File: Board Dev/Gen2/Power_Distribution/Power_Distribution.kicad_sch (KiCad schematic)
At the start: 27 parts, among them IC1 ACS713ELCTR-30A-T, IC2 ACS713ELCTR-30A-T, IC3 ACS713ELCTR-30A-T, IC4 ACS713ELCTR-30A-T, IC5 ACS713ELCTR-30A-T, IC6 ACS713ELCTR-30A-T, IC7 ACS713ELCTR-30A-T, IC8 ACS713ELCTR-30A-T, J1 8TERM_VERT_1719370, J2 8TERM_VERT_1719370, J3 Conn_01x02_Socket

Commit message: Final Power Dist Board
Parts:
- removed J3: Conn_01x02_Socket, symbol Connector:Conn_01x02_Socket
- added J3, J5: Conn_01x04_Socket, Connector_PinHeader_2.54mm:PinHeader_1x04_P2.54mm_Vertical, symbol Connector:Conn_01x04_Socket
- added J4: 1986660-2, CONN2_1986660-2_TEC, symbol HighPowerRoboConnector:1986660-2
- C_byp1, C_byp2, C_byp3, C_byp4, C_byp5, C_byp6, C_byp7, C_byp8: footprint (none) -> Capacitor_SMD:C_0805_2012Metric_Pad1.18x1.45mm_HandSolder
- C_filter1, C_filter2, C_filter3, C_filter4, C_filter5, C_filter6, C_filter7, C_filter8: footprint 0802 cap:0802 Cap -> Capacitor_SMD:C_0805_2012Metric_Pad1.18x1.45mm_HandSolder
- IC2, IC3, IC4, IC5, IC6, IC7: footprint Imported_Footprints:ACS711ELCTR25ABT -> Imported_Footprints:MyHalleffectSensor
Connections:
- net +BATT: now also J4.1A, J4.1B
- net -BATT: now also J4.2A, J4.2B
- net VIout1: now also J3.4 (Pin_4)
- net VIout2: now also J3.3 (Pin_3)
- net VIout3: now also J3.2 (Pin_2)
- net VIout4: now also J3.1 (Pin_1)
- net VIout5: now also J5.4 (Pin_4)
- net VIout6: now also J5.3 (Pin_3)
- net VIout7: now also J5.2 (Pin_2)
- net VIout8: now also J5.1 (Pin_1)
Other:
- note added: "Connectors To ESCs"
- note added: "Hall Effect Sensors"
- note added: "High Power Connector Socket For Bat in and Gnd"
- note added: "One by Four Pin Headers"
- moved on the sheet: J1, J2

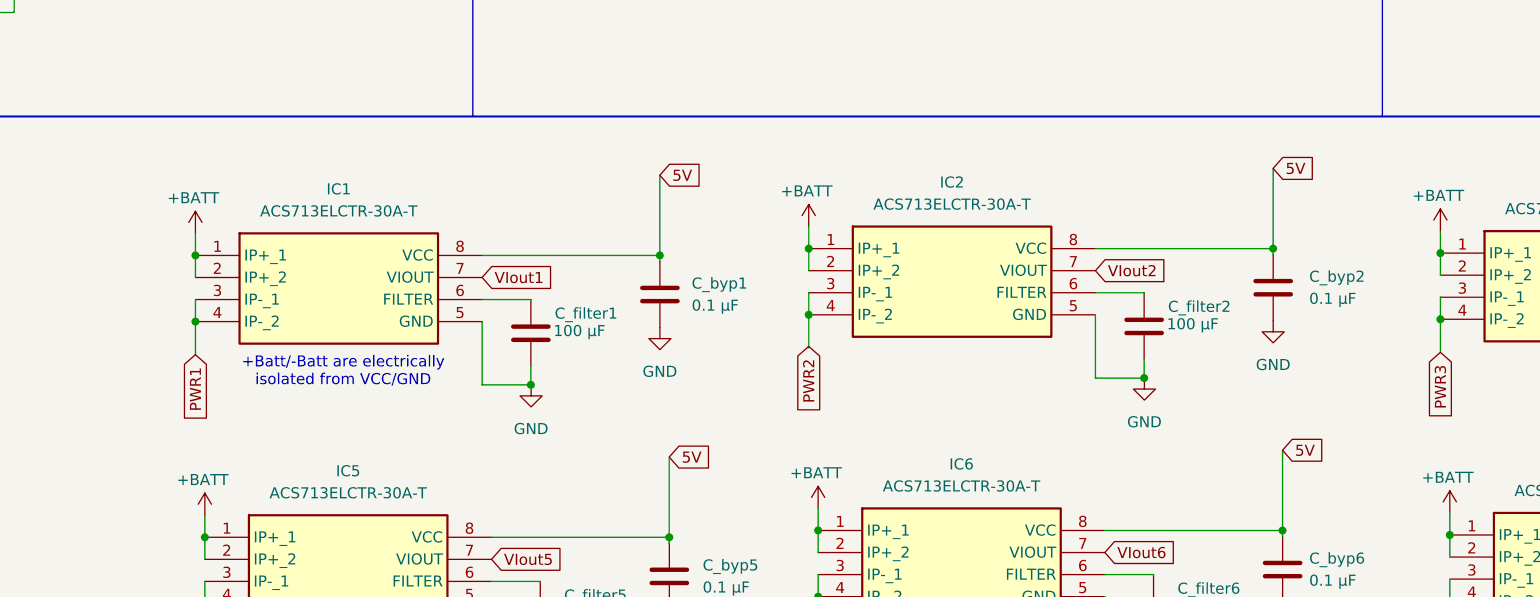
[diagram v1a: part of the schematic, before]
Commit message: good spot
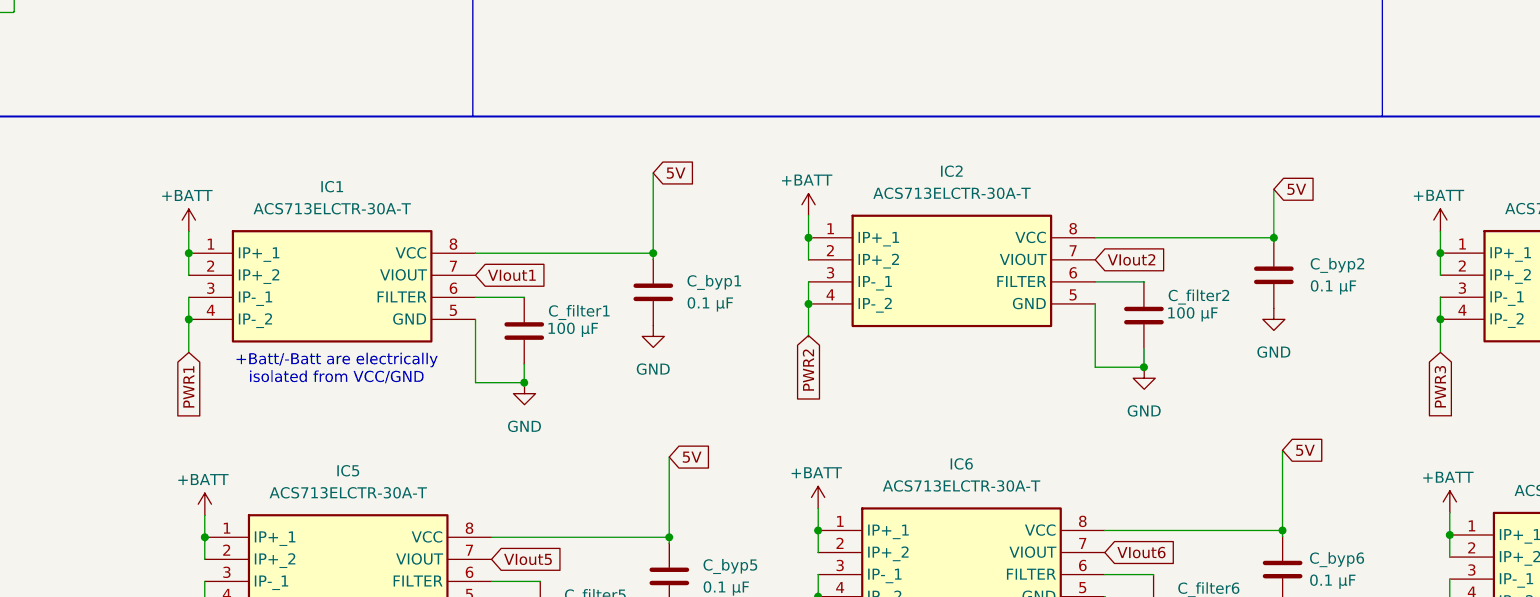
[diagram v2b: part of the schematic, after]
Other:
- moved on the sheet: C_byp2, C_filter1, C_filter2, IC1, IC2
